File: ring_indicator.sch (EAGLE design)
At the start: 21 parts, among them Q2 BUZ11

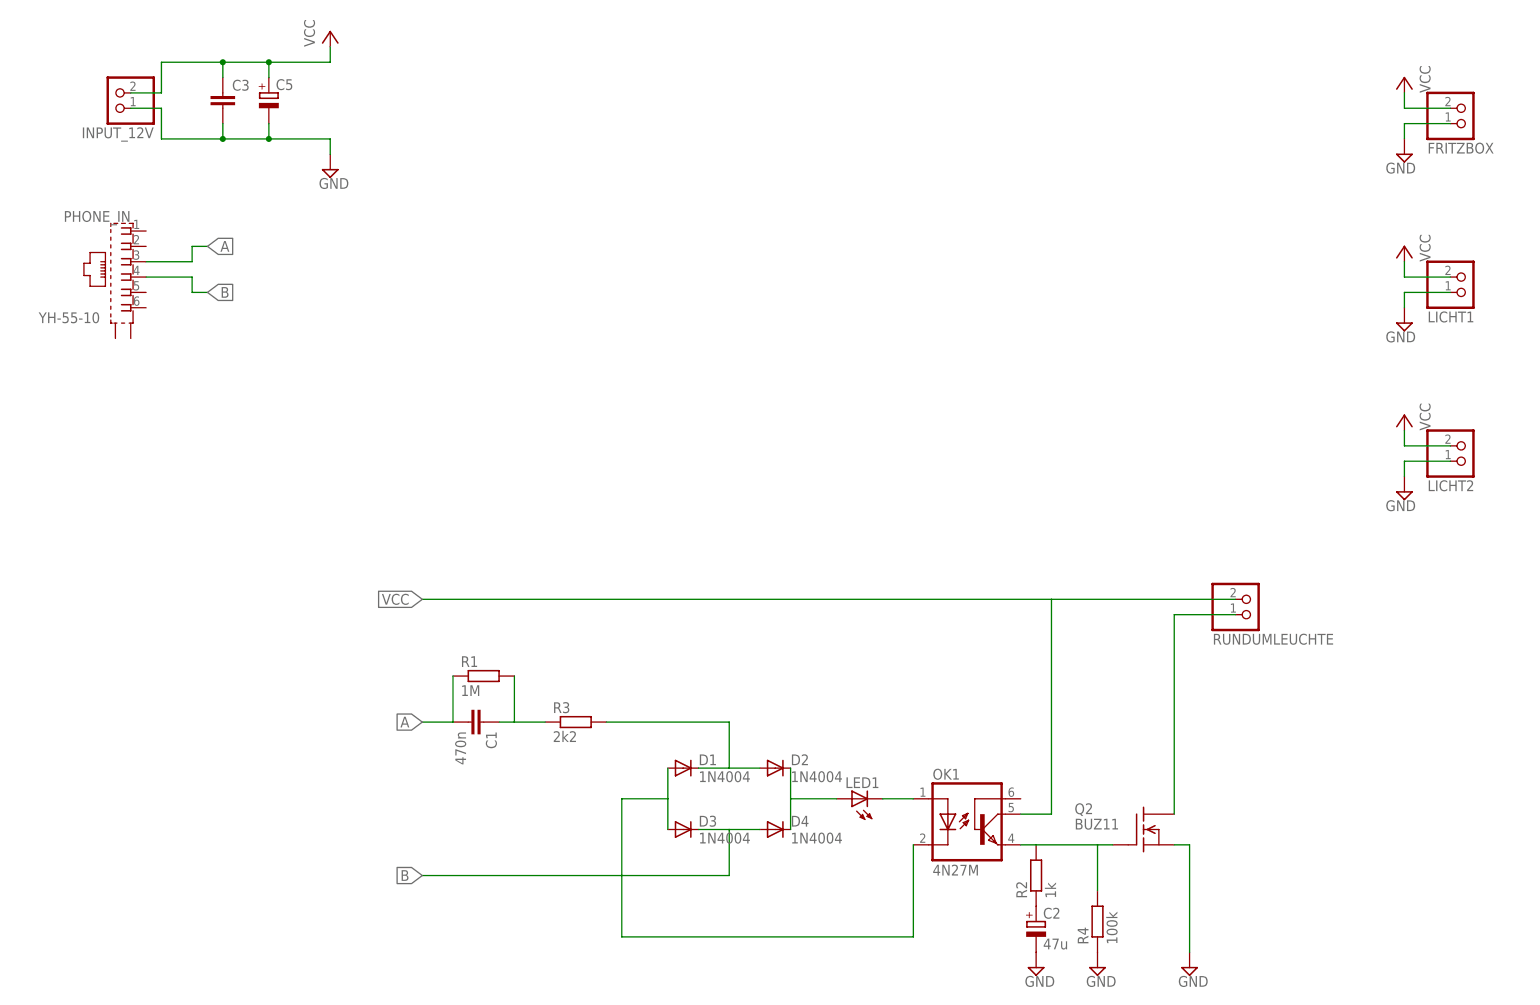
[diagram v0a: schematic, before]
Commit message: v0.2-produced
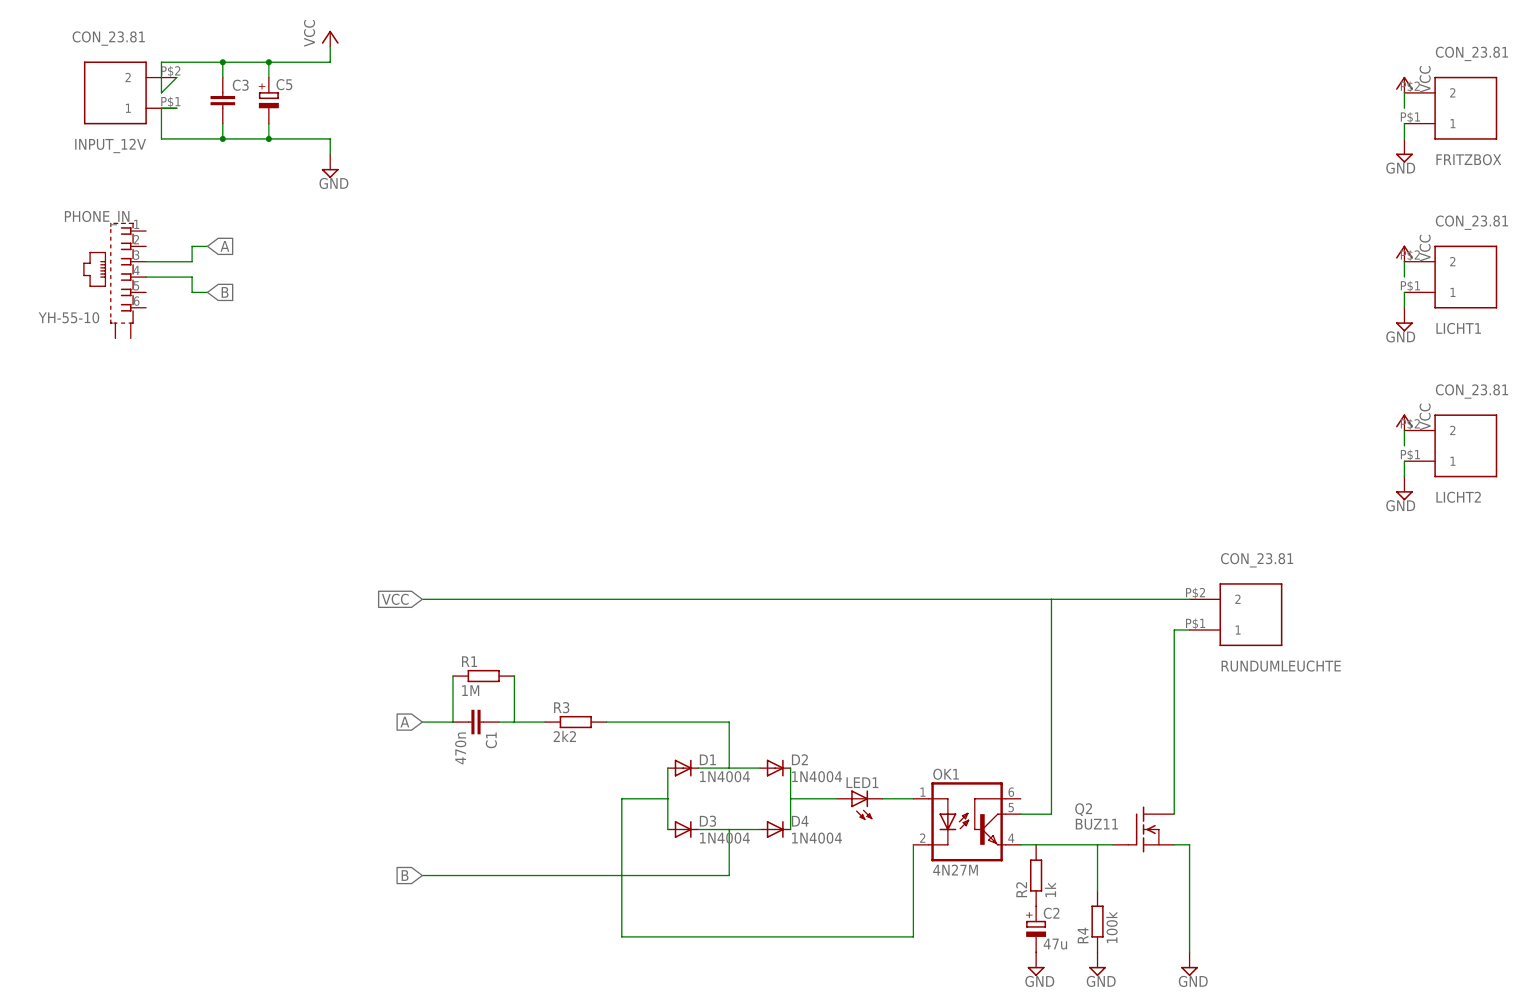
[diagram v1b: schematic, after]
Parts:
- FRITZBOX, INPUT_12V, LICHT1, LICHT2, RUNDUMLEUCHTE: value (none) -> CON_23.81; device pinhead:PINHD-1X2 -> pcaroli:CON_23.81
- R1, R2, R3, R4: device rcl:R-EU_0204/5 -> rcl:R-EU_0207/10
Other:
- moved on the sheet: FRITZBOX, INPUT_12V, LICHT1, LICHT2, RUNDUMLEUCHTE
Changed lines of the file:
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@@
 <layer number="51" name="tDocu" color="6" fill="1" visible="no" active="no"/>
 <layer number="52" name="bDocu" color="7" fill="1" visible="no" active="no"/>
+<layer number="90" name="Modules" color="5" fill="1" visible="yes" active="yes"/>
 <layer number="91" name="Nets" color="2" fill="1" visible="yes" active="yes"/>
 <layer number="92" name="Busses" color="1" fill="1" visible="yes" active="yes"/>
@@
 <parts>
 <part name="PHONE_IN" library="con-wenzhou-yihua" deviceset="YH-55-10" device=""/>
-<part name="FRITZBOX" library="pinhead" deviceset="PINHD-1X2" device=""/>
-<part name="LICHT1" library="pinhead" deviceset="PINHD-1X2" device=""/>
-<part name="LICHT2" library="pinhead" deviceset="PINHD-1X2" device=""/>
-<part name="RUNDUMLEUCHTE" library="pinhead" deviceset="PINHD-1X2" device=""/>
+<part name="FRITZBOX" library="pcaroli" deviceset="CON_2" device="3.81"/>
+<part name="LICHT1" library="pcaroli" deviceset="CON_2" device="3.81"/>
+<part name="LICHT2" library="pcaroli" deviceset="CON_2" device="3.81"/>
+<part name="RUNDUMLEUCHTE" library="pcaroli" deviceset="CON_2" device="3.81"/>
 <part name="SUPPLY1" library="supply2" deviceset="GND" device=""/>
 <part name="P+1" library="supply1" deviceset="VCC" device=""/>
@@
 <part name="SUPPLY2" library="supply2" deviceset="GND" device=""/>
 <part name="SUPPLY3" library="supply2" deviceset="GND" device=""/>
-<part name="INPUT_12V" library="pinhead" deviceset="PINHD-1X2" device=""/>
+<part name="INPUT_12V" library="pcaroli" deviceset="CON_2" device="3.81"/>
 <part name="SUPPLY4" library="supply2" deviceset="GND" device=""/>
 <part name="P+4" library="supply1" deviceset="VCC" device=""/>
 <part name="C1" library="resistor" deviceset="C-EU" device="102-064X133" value="470n"/>
 <part name="C2" library="rcl" deviceset="CPOL-EU" device="E3.5-8" value="47u"/>
-<part name="R1" library="rcl" deviceset="R-EU_" device="0204/5" value="1M"/>
-<part name="R2" library="rcl" deviceset="R-EU_" device="0204/5" value="1k"/>
+<part name="R1" library="rcl" deviceset="R-EU_" device="0207/10" value="1M"/>
+<part name="R2" library="rcl" deviceset="R-EU_" device="0207/10" value="1k"/>
 <part name="D1" library="diode" deviceset="1N4004" device=""/>
 <part name="D2" library="diode" deviceset="1N4004" device=""/>
 <part name="D3" library="diode" deviceset="1N4004" device=""/>
 <part name="D4" library="diode" deviceset="1N4004" device=""/>
-<part name="R3" library="rcl" deviceset="R-EU_" device="0204/5" value="2k2"/>
+<part name="R3" library="rcl" deviceset="R-EU_" device="0207/10" value="2k2"/>
 <part name="LED1" library="led" deviceset="LED" device="5MM"/>
-<part name="R4" library="rcl" deviceset="R-EU_" device="0204/5" value="100k"/>
+<part name="R4" library="rcl" deviceset="R-EU_" device="0207/10" value="100k"/>
 <part name="OK1" library="optocoupler" deviceset="4N*?M" device="" technology="27"/>
 <part name="Q2" library="transistor-fet" deviceset="BUZ11" device=""/>
@@
 <instance part="LICHT1" gate="G$1" x="256.54" y="88.9" rot="MR180"/>
 <instance part="LICHT2" gate="G$1" x="256.54" y="60.96" rot="MR180"/>
-<instance part="RUNDUMLEUCHTE" gate="G$1" x="220.98" y="35.56" rot="MR180"/>
+<instance part="RUNDUMLEUCHTE" gate="G$1" x="220.98" y="33.02" rot="MR180"/>
 <instance part="SUPPLY1" gate="GND" x="246.38" y="109.22" rot="MR0"/>
 <instance part="P+1" gate="VCC" x="246.38" y="121.92" rot="MR0"/>
@@
 <segment>
 <pinref part="FRITZBOX" gate="G$1" pin="1"/>
-<wire x1="254" y1="114.3" x2="246.38" y2="114.3" width="0.1524" layer="91"/>
 <wire x1="246.38" y1="114.3" x2="246.38" y2="111.76" width="0.1524" layer="91"/>
 <pinref part="SUPPLY1" gate="GND" pin="GND"/>
@@
 <segment>
 <pinref part="LICHT1" gate="G$1" pin="1"/>
-<wire x1="254" y1="86.36" x2="246.38" y2="86.36" width="0.1524" layer="91"/>
 <wire x1="246.38" y1="86.36" x2="246.38" y2="83.82" width="0.1524" layer="91"/>
 <pinref part="SUPPLY2" gate="GND" pin="GND"/>
@@
 <segment>
 <pinref part="LICHT2" gate="G$1" pin="1"/>
-<wire x1="254" y1="58.42" x2="246.38" y2="58.42" width="0.1524" layer="91"/>
 <wire x1="246.38" y1="58.42" x2="246.38" y2="55.88" width="0.1524" layer="91"/>
 <pinref part="SUPPLY3" gate="GND" pin="GND"/>
@@
 <wire x1="68.58" y1="111.76" x2="68.58" y2="109.22" width="0.1524" layer="91"/>
 <pinref part="INPUT_12V" gate="G$1" pin="1"/>
-<wire x1="35.56" y1="116.84" x2="40.64" y2="116.84" width="0.1524" layer="91"/>
+<wire x1="43.18" y1="116.84" x2="40.64" y2="116.84" width="0.1524" layer="91"/>
 <wire x1="40.64" y1="116.84" x2="40.64" y2="111.76" width="0.1524" layer="91"/>
 <wire x1="40.64" y1="111.76" x2="50.8" y2="111.76" width="0.1524" layer="91"/>
@@
 <segment>
 <pinref part="FRITZBOX" gate="G$1" pin="2"/>
-<wire x1="254" y1="116.84" x2="246.38" y2="116.84" width="0.1524" layer="91"/>
 <wire x1="246.38" y1="116.84" x2="246.38" y2="119.38" width="0.1524" layer="91"/>
 <pinref part="P+1" gate="VCC" pin="VCC"/>
@@
 <segment>
 <pinref part="LICHT1" gate="G$1" pin="2"/>
-<wire x1="254" y1="88.9" x2="246.38" y2="88.9" width="0.1524" layer="91"/>
 <wire x1="246.38" y1="88.9" x2="246.38" y2="91.44" width="0.1524" layer="91"/>
 <pinref part="P+2" gate="VCC" pin="VCC"/>
@@
 <segment>
 <pinref part="LICHT2" gate="G$1" pin="2"/>
-<wire x1="254" y1="60.96" x2="246.38" y2="60.96" width="0.1524" layer="91"/>
 <wire x1="246.38" y1="60.96" x2="246.38" y2="63.5" width="0.1524" layer="91"/>
 <pinref part="P+3" gate="VCC" pin="VCC"/>
@@
 <pinref part="RUNDUMLEUCHTE" gate="G$1" pin="2"/>
 <pinref part="OK1" gate="G$1" pin="COL"/>
-<wire x1="187.96" y1="35.56" x2="218.44" y2="35.56" width="0.1524" layer="91"/>
+<wire x1="187.96" y1="35.56" x2="210.82" y2="35.56" width="0.1524" layer="91"/>
 <wire x1="182.88" y1="0" x2="187.96" y2="0" width="0.1524" layer="91"/>
 <wire x1="187.96" y1="0" x2="187.96" y2="35.56" width="0.1524" layer="91"/>
@@
 <wire x1="68.58" y1="124.46" x2="68.58" y2="127" width="0.1524" layer="91"/>
 <pinref part="INPUT_12V" gate="G$1" pin="2"/>
-<wire x1="35.56" y1="119.38" x2="40.64" y2="119.38" width="0.1524" layer="91"/>
+<wire x1="43.18" y1="121.92" x2="40.64" y2="119.38" width="0.1524" layer="91"/>
 <wire x1="40.64" y1="119.38" x2="40.64" y2="124.46" width="0.1524" layer="91"/>
 <wire x1="40.64" y1="124.46" x2="50.8" y2="124.46" width="0.1524" layer="91"/>
@@
 <segment>
 <pinref part="RUNDUMLEUCHTE" gate="G$1" pin="1"/>
-<wire x1="218.44" y1="33.02" x2="208.28" y2="33.02" width="0.1524" layer="91"/>
+<wire x1="210.82" y1="30.48" x2="208.28" y2="30.48" width="0.1524" layer="91"/>
 <pinref part="Q2" gate="G$1" pin="D"/>
-<wire x1="208.28" y1="0" x2="208.28" y2="33.02" width="0.1524" layer="91"/>
-</segment>
-</net>
+<wire x1="208.28" y1="0" x2="208.28" y2="30.48" width="0.1524" layer="91"/>
+</segment>
+</net>

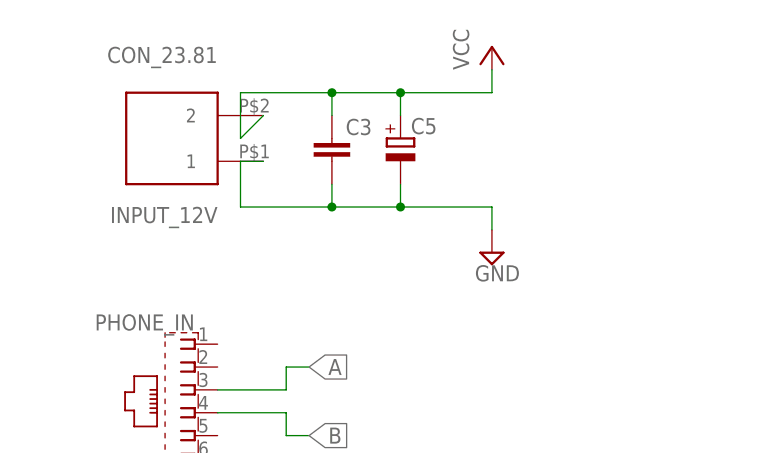
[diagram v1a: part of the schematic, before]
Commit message: v0.2.1-cleanup
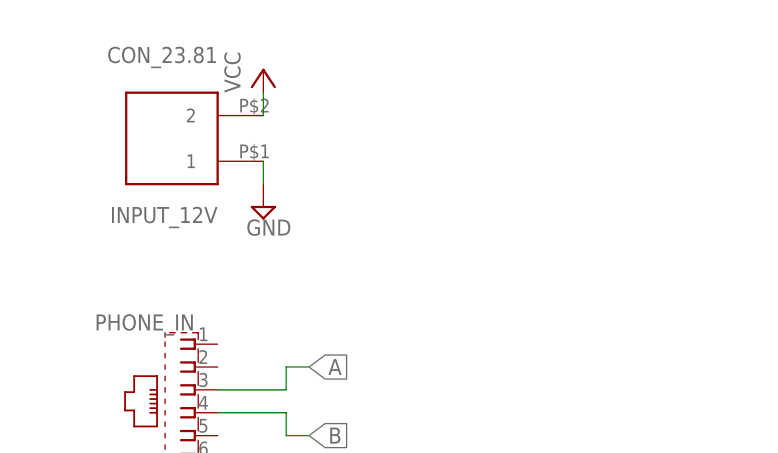
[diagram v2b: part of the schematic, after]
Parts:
- removed C3: (no value), capacitor-wima:C2,5-3
- removed C5: (no value), resistor:CPOL-EUTT2D6
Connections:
- net GND: no longer C3.2, C5.-
- net VCC: no longer C3.1, C5.+
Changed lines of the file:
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@@
 <part name="SUPPLY6" library="supply2" deviceset="GND" device=""/>
 <part name="SUPPLY7" library="supply2" deviceset="GND" device=""/>
-<part name="C3" library="capacitor-wima" deviceset="C" device="2,5-3"/>
-<part name="C5" library="resistor" deviceset="CPOL-EU" device="TT2D6"/>
 </parts>
 <sheets>
@@
 <instance part="SUPPLY3" gate="GND" x="246.38" y="53.34" rot="MR0"/>
 <instance part="INPUT_12V" gate="G$1" x="33.02" y="119.38" rot="R180"/>
-<instance part="SUPPLY4" gate="GND" x="68.58" y="106.68"/>
-<instance part="P+4" gate="VCC" x="68.58" y="129.54"/>
+<instance part="SUPPLY4" gate="GND" x="43.18" y="111.76"/>
+<instance part="P+4" gate="VCC" x="43.18" y="127"/>
 <instance part="C1" gate="G$1" x="93.98" y="15.24" rot="R270"/>
 <instance part="C2" gate="G$1" x="185.42" y="-17.78"/>
@@
 <instance part="SUPPLY6" gate="GND" x="185.42" y="-25.4"/>
 <instance part="SUPPLY7" gate="GND" x="210.82" y="-25.4"/>
-<instance part="C3" gate="G$1" x="50.8" y="119.38"/>
-<instance part="C5" gate="G$1" x="58.42" y="119.38"/>
 </instances>
 <busses>
@@
 </segment>
 <segment>
+<pinref part="INPUT_12V" gate="G$1" pin="1"/>
 <pinref part="SUPPLY4" gate="GND" pin="GND"/>
-<wire x1="68.58" y1="111.76" x2="68.58" y2="109.22" width="0.1524" layer="91"/>
-<pinref part="INPUT_12V" gate="G$1" pin="1"/>
-<wire x1="43.18" y1="116.84" x2="40.64" y2="116.84" width="0.1524" layer="91"/>
-<wire x1="40.64" y1="116.84" x2="40.64" y2="111.76" width="0.1524" layer="91"/>
-<wire x1="40.64" y1="111.76" x2="50.8" y2="111.76" width="0.1524" layer="91"/>
-<wire x1="50.8" y1="111.76" x2="58.42" y2="111.76" width="0.1524" layer="91"/>
-<wire x1="58.42" y1="111.76" x2="68.58" y2="111.76" width="0.1524" layer="91"/>
-<wire x1="58.42" y1="111.76" x2="58.42" y2="114.3" width="0.1524" layer="91"/>
-<junction x="58.42" y="111.76"/>
-<pinref part="C3" gate="G$1" pin="2"/>
-<wire x1="50.8" y1="111.76" x2="50.8" y2="114.3" width="0.1524" layer="91"/>
-<junction x="50.8" y="111.76"/>
-<pinref part="C5" gate="G$1" pin="-"/>
+<wire x1="43.18" y1="116.84" x2="43.18" y2="114.3" width="0.1524" layer="91"/>
 </segment>
 </net>
@@
 </segment>
 <segment>
+<pinref part="INPUT_12V" gate="G$1" pin="2"/>
+<wire x1="43.18" y1="121.92" x2="43.18" y2="124.46" width="0.1524" layer="91"/>
 <pinref part="P+4" gate="VCC" pin="VCC"/>
-<wire x1="68.58" y1="124.46" x2="68.58" y2="127" width="0.1524" layer="91"/>
-<pinref part="INPUT_12V" gate="G$1" pin="2"/>
-<wire x1="43.18" y1="121.92" x2="40.64" y2="119.38" width="0.1524" layer="91"/>
-<wire x1="40.64" y1="119.38" x2="40.64" y2="124.46" width="0.1524" layer="91"/>
-<wire x1="40.64" y1="124.46" x2="50.8" y2="124.46" width="0.1524" layer="91"/>
-<wire x1="50.8" y1="124.46" x2="58.42" y2="124.46" width="0.1524" layer="91"/>
-<wire x1="58.42" y1="124.46" x2="68.58" y2="124.46" width="0.1524" layer="91"/>
-<wire x1="58.42" y1="124.46" x2="58.42" y2="121.92" width="0.1524" layer="91"/>
-<junction x="58.42" y="124.46"/>
-<pinref part="C3" gate="G$1" pin="1"/>
-<wire x1="50.8" y1="124.46" x2="50.8" y2="121.92" width="0.1524" layer="91"/>
-<junction x="50.8" y="124.46"/>
-<pinref part="C5" gate="G$1" pin="+"/>
 </segment>
 </net>
